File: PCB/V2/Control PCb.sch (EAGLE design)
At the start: 33 parts, among them Q1 DMP2305U-7, Q2 BSS123, Q3 BSS123, U1 V_REG_317DPACK, U2 5ACFEW

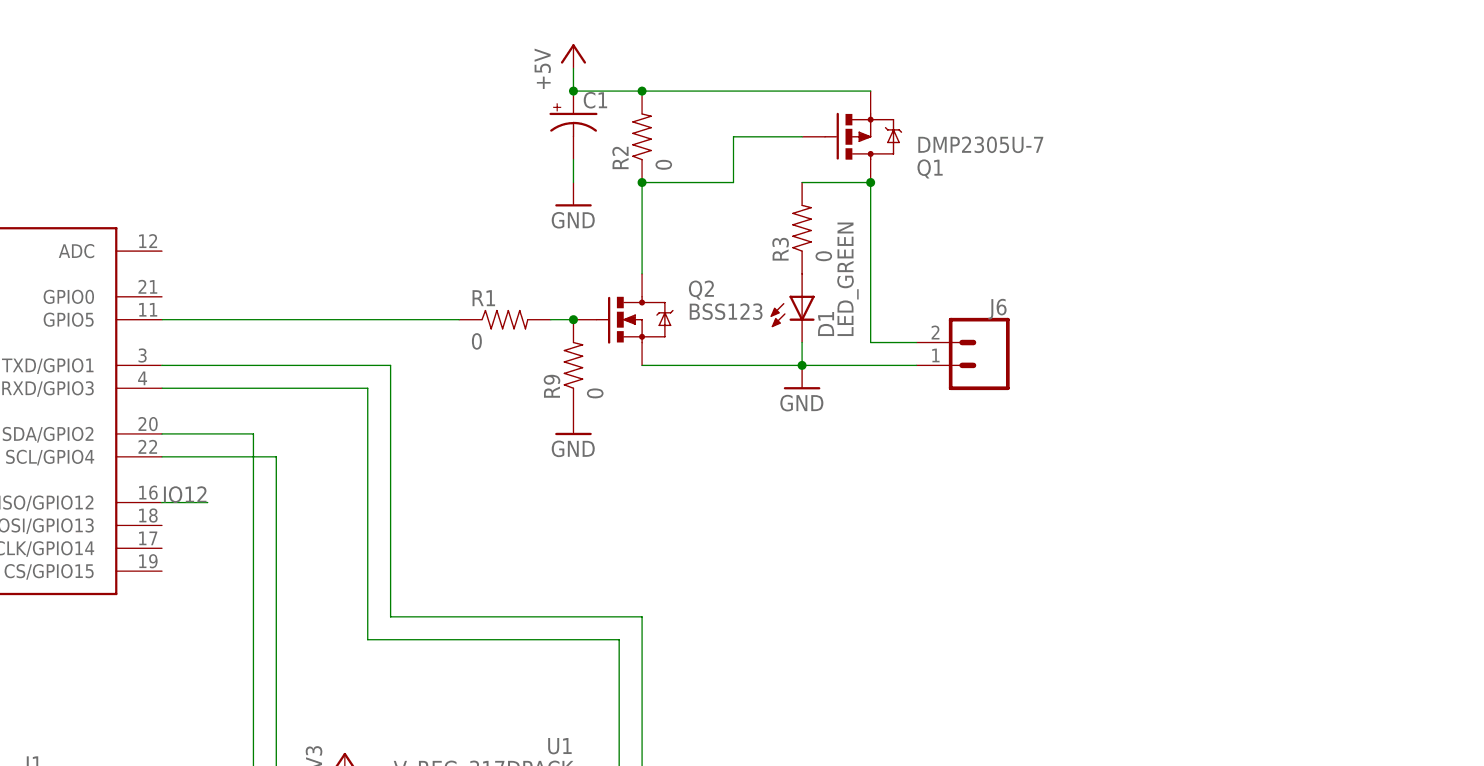
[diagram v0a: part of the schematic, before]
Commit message: Code + PCB stuff
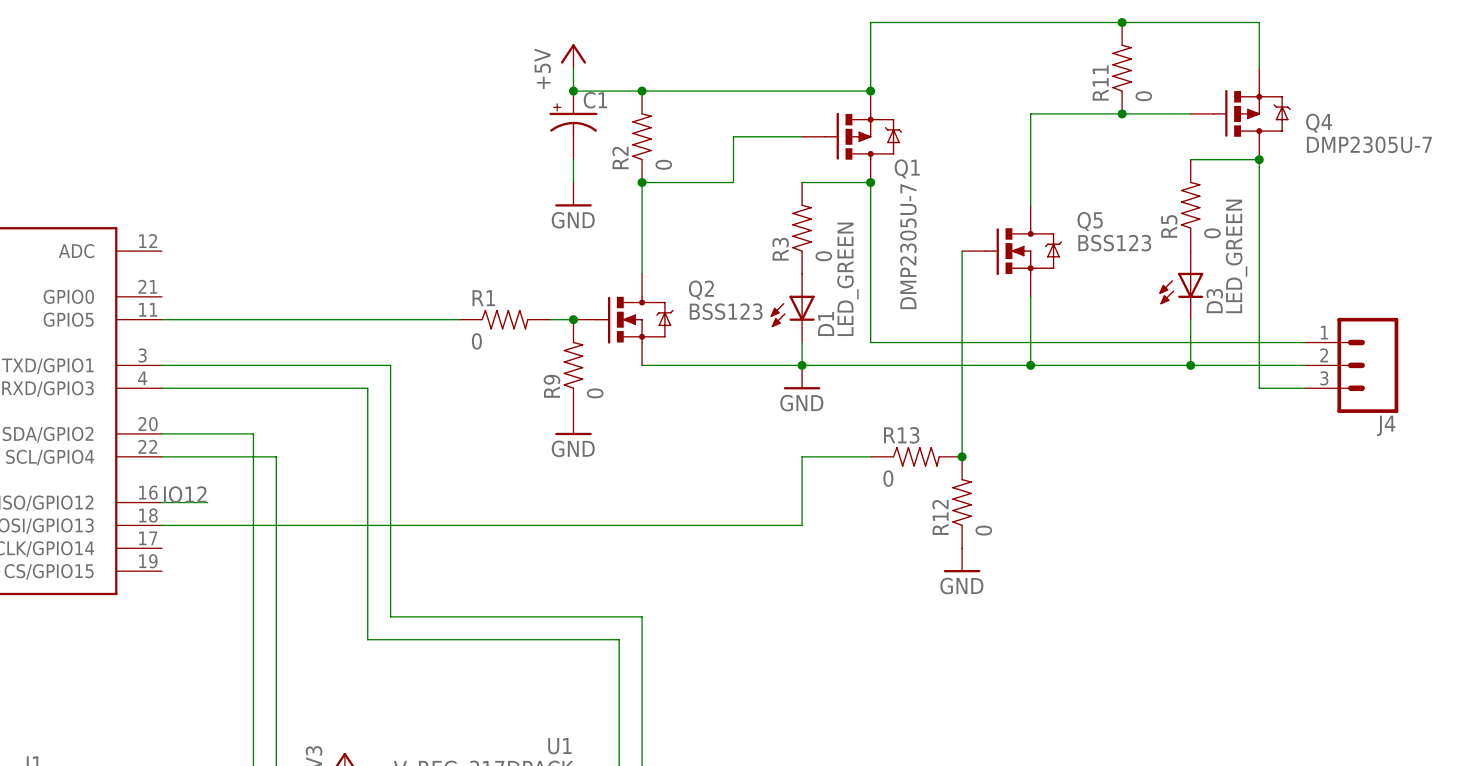
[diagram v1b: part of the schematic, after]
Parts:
- removed J6: (no value), SparkFun-Connectors:CONN_025MM
- added D3: LED_GREEN, RJC-2:LED_GREEN
- added J4: (no value), SparkFun-Connectors:CONN_03-SCREW-5MM
- added Q4: DMP2305U-7, RJC-2:MOS-P_DMP2305U-7
- added Q5: BSS123, RJC-2:MOS-N_BSS123
- added R11, R12, R13, R5: 0, RJC-2:RES_0_0805
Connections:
- new net N$16: J4.3, Q4.D, R5.2
- new net N$19: D3.A, R5.1
- new net N$20: Q4.G, Q5.D, R11.1
- new net N$21: R13.1, U$1.MOSI/GPIO13
- new net N$22: Q5.G, R12.2, R13.2
- net +5V: now also Q4.S, R11.2
- net GND: now also D3.C, J4.2, Q5.S, R12.1; no longer J6.1
- net N$6: now also J4.1; no longer J6.2
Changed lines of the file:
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@@
 <part name="GND6" library="supply1" library_urn="urn:adsk.eagle:library:371" deviceset="GND" device=""/>
 <part name="GND7" library="supply1" library_urn="urn:adsk.eagle:library:371" deviceset="GND" device=""/>
-<part name="J6" library="SparkFun-Connectors" library_urn="urn:adsk.eagle:library:513" deviceset="CONN_02" device="5MM" package3d_urn="urn:adsk.eagle:package:38044/1"/>
 <part name="R9" library="RJC-2" library_urn="urn:adsk.eagle:library:33162582" deviceset="RES" device="_0_0805" package3d_urn="urn:adsk.eagle:package:33163805/3" value="0"/>
 <part name="GND8" library="supply1" library_urn="urn:adsk.eagle:library:371" deviceset="GND" device=""/>
@@
 <part name="C2" library="SparkFun-Capacitors" library_urn="urn:adsk.eagle:library:510" deviceset="1000UF" device="-RADIAL-5MM-35V-20%-KIT" package3d_urn="urn:adsk.eagle:package:37421/1" value="470"/>
 <part name="C5" library="SparkFun-Capacitors" library_urn="urn:adsk.eagle:library:510" deviceset="1000UF" device="-RADIAL-5MM-35V-20%-KIT" package3d_urn="urn:adsk.eagle:package:37421/1" value="100"/>
+<part name="J4" library="SparkFun-Connectors" library_urn="urn:adsk.eagle:library:513" deviceset="CONN_03" device="-SCREW-5MM" package3d_urn="urn:adsk.eagle:package:38070/1"/>
+<part name="Q4" library="RJC-2" library_urn="urn:adsk.eagle:library:33162582" deviceset="MOS-P" device="_DMP2305U-7" package3d_urn="urn:adsk.eagle:package:33163661/2" value="DMP2305U-7"/>
+<part name="R5" library="RJC-2" library_urn="urn:adsk.eagle:library:33162582" deviceset="RES" device="_0_0805" package3d_urn="urn:adsk.eagle:package:33163805/3" value="0"/>
+<part name="D3" library="RJC-2" library_urn="urn:adsk.eagle:library:33162582" deviceset="LED" device="_GREEN" package3d_urn="urn:adsk.eagle:package:33163857/2"/>
+<part name="R11" library="RJC-2" library_urn="urn:adsk.eagle:library:33162582" deviceset="RES" device="_0_0805" package3d_urn="urn:adsk.eagle:package:33163805/3" value="0"/>
+<part name="Q5" library="RJC-2" library_urn="urn:adsk.eagle:library:33162582" deviceset="MOS-N" device="_BSS123" package3d_urn="urn:adsk.eagle:package:33163661/2" value="BSS123"/>
+<part name="R12" library="RJC-2" library_urn="urn:adsk.eagle:library:33162582" deviceset="RES" device="_0_0805" package3d_urn="urn:adsk.eagle:package:33163805/3" value="0"/>
+<part name="R13" library="RJC-2" library_urn="urn:adsk.eagle:library:33162582" deviceset="RES" device="_0_0805" package3d_urn="urn:adsk.eagle:package:33163805/3" value="0"/>
+<part name="GND10" library="supply1" library_urn="urn:adsk.eagle:library:371" deviceset="GND" device=""/>
 </parts>
 <sheets>
@@
 </instance>
 <instance part="Q1" gate="G$1" x="119.38" y="96.52" smashed="yes" rot="MR180">
-<attribute name="NAME" x="124.46" y="93.98" size="1.778" layer="95" rot="MR180"/>
-<attribute name="VALUE" x="124.46" y="96.52" size="1.778" layer="96" rot="MR180"/>
+<attribute name="NAME" x="121.92" y="93.98" size="1.778" layer="95" rot="MR180"/>
+<attribute name="VALUE" x="124.46" y="91.44" size="1.778" layer="96" rot="MR270"/>
 </instance>
 <instance part="Q2" gate="G$1" x="93.98" y="76.2" smashed="yes">
@@
 <attribute name="VALUE" x="109.22" y="66.04" size="1.778" layer="96"/>
 </instance>
-<instance part="J6" gate="G$1" x="132.08" y="71.12" smashed="yes" rot="MR0">
-<attribute name="VALUE" x="134.62" y="66.294" size="1.778" layer="96" font="vector" rot="MR0"/>
-<attribute name="NAME" x="134.62" y="76.708" size="1.778" layer="95" font="vector" rot="MR0"/>
-</instance>
 <instance part="R9" gate="G$1" x="86.36" y="71.12" smashed="yes" rot="R90">
 <attribute name="NAME" x="84.8614" y="67.31" size="1.778" layer="95" rot="R90"/>
@@
 <attribute name="NAME" x="89.916" y="-17.145" size="1.778" layer="95" font="vector"/>
 <attribute name="VALUE" x="89.916" y="-21.971" size="1.778" layer="96" font="vector"/>
+</instance>
+<instance part="J4" gate="J$1" x="175.26" y="71.12" smashed="yes" rot="R180">
+<attribute name="VALUE" x="177.8" y="78.486" size="1.778" layer="96" font="vector" rot="R180"/>
+<attribute name="NAME" x="177.8" y="65.532" size="1.778" layer="95" font="vector" rot="R180"/>
+</instance>
+<instance part="Q4" gate="G$1" x="162.56" y="99.06" smashed="yes" rot="MR180">
+<attribute name="NAME" x="167.64" y="99.06" size="1.778" layer="95" rot="MR180"/>
+<attribute name="VALUE" x="167.64" y="96.52" size="1.778" layer="96" rot="MR180"/>
+</instance>
+<instance part="R5" gate="G$1" x="154.94" y="88.9" smashed="yes" rot="R90">
+<attribute name="NAME" x="153.4414" y="85.09" size="1.778" layer="95" rot="R90"/>
+<attribute name="VALUE" x="158.242" y="85.09" size="1.778" layer="96" rot="R90"/>
+</instance>
+<instance part="D3" gate="G$1" x="154.94" y="78.74" smashed="yes">
+<attribute name="NAME" x="158.496" y="76.708" size="1.778" layer="95" rot="R90"/>
+<attribute name="VALUE" x="160.655" y="76.708" size="1.778" layer="96" rot="R90"/>
+</instance>
+<instance part="R11" gate="G$1" x="147.32" y="104.14" smashed="yes" rot="R90">
+<attribute name="NAME" x="145.8214" y="100.33" size="1.778" layer="95" rot="R90"/>
+<attribute name="VALUE" x="150.622" y="100.33" size="1.778" layer="96" rot="R90"/>
+</instance>
+<instance part="Q5" gate="G$1" x="137.16" y="83.82" smashed="yes">
+<attribute name="NAME" x="142.24" y="86.36" size="1.778" layer="95"/>
+<attribute name="VALUE" x="142.24" y="83.82" size="1.778" layer="96"/>
+</instance>
+<instance part="R12" gate="G$1" x="129.54" y="55.88" smashed="yes" rot="R90">
+<attribute name="NAME" x="128.0414" y="52.07" size="1.778" layer="95" rot="R90"/>
+<attribute name="VALUE" x="132.842" y="52.07" size="1.778" layer="96" rot="R90"/>
+</instance>
+<instance part="R13" gate="G$1" x="124.46" y="60.96" smashed="yes">
+<attribute name="NAME" x="120.65" y="62.4586" size="1.778" layer="95"/>
+<attribute name="VALUE" x="120.65" y="57.658" size="1.778" layer="96"/>
+</instance>
+<instance part="GND10" gate="1" x="129.54" y="48.26" smashed="yes">
+<attribute name="VALUE" x="127" y="45.72" size="1.778" layer="96"/>
 </instance>
 </instances>
@@
 <junction x="111.76" y="71.12"/>
 <pinref part="GND7" gate="1" pin="GND"/>
-<pinref part="J6" gate="G$1" pin="1"/>
-<wire x1="124.46" y1="71.12" x2="111.76" y2="71.12" width="0.1524" layer="91"/>
+<wire x1="167.64" y1="71.12" x2="154.94" y2="71.12" width="0.1524" layer="91"/>
+<pinref part="J4" gate="J$1" pin="2"/>
+<pinref part="D3" gate="G$1" pin="C"/>
+<wire x1="154.94" y1="71.12" x2="137.16" y2="71.12" width="0.1524" layer="91"/>
+<wire x1="137.16" y1="71.12" x2="111.76" y2="71.12" width="0.1524" layer="91"/>
+<wire x1="154.94" y1="76.2" x2="154.94" y2="71.12" width="0.1524" layer="91"/>
+<junction x="154.94" y="71.12"/>
+<pinref part="Q5" gate="G$1" pin="S"/>
+<wire x1="137.16" y1="78.74" x2="137.16" y2="71.12" width="0.1524" layer="91"/>
+<junction x="137.16" y="71.12"/>
 </segment>
 <segment>
@@
 <pinref part="GND9" gate="1" pin="GND"/>
 <wire x1="-7.62" y1="81.28" x2="-7.62" y2="78.74" width="0.1524" layer="91"/>
+</segment>
+<segment>
+<pinref part="R12" gate="G$1" pin="1"/>
+<pinref part="GND10" gate="1" pin="GND"/>
 </segment>
 </net>
@@
 <wire x1="93.98" y1="101.6" x2="119.38" y2="101.6" width="0.1524" layer="91"/>
 <junction x="93.98" y="101.6"/>
+<wire x1="119.38" y1="101.6" x2="119.38" y2="109.22" width="0.1524" layer="91"/>
+<wire x1="119.38" y1="109.22" x2="147.32" y2="109.22" width="0.1524" layer="91"/>
+<junction x="119.38" y="101.6"/>
+<pinref part="Q4" gate="G$1" pin="S"/>
+<wire x1="147.32" y1="109.22" x2="162.56" y2="109.22" width="0.1524" layer="91"/>
+<wire x1="162.56" y1="109.22" x2="162.56" y2="104.14" width="0.1524" layer="91"/>
+<pinref part="R11" gate="G$1" pin="2"/>
+<junction x="147.32" y="109.22"/>
 </segment>
 <segment>
@@
 <wire x1="119.38" y1="91.44" x2="119.38" y2="73.66" width="0.1524" layer="91"/>
 <junction x="119.38" y="91.44"/>
-<pinref part="J6" gate="G$1" pin="2"/>
-<wire x1="119.38" y1="73.66" x2="124.46" y2="73.66" width="0.1524" layer="91"/>
+<wire x1="119.38" y1="73.66" x2="167.64" y2="73.66" width="0.1524" layer="91"/>
+<pinref part="J4" gate="J$1" pin="1"/>
 </segment>
 </net>
@@
 </segment>
 </net>
+<net name="N$16" class="0">
+<segment>
+<pinref part="Q4" gate="G$1" pin="D"/>
+<wire x1="162.56" y1="93.98" x2="162.56" y2="68.58" width="0.1524" layer="91"/>
+<pinref part="J4" gate="J$1" pin="3"/>
+<wire x1="162.56" y1="68.58" x2="167.64" y2="68.58" width="0.1524" layer="91"/>
+<pinref part="R5" gate="G$1" pin="2"/>
+<wire x1="154.94" y1="93.98" x2="162.56" y2="93.98" width="0.1524" layer="91"/>
+<junction x="162.56" y="93.98"/>
+</segment>
+</net>
+<net name="N$19" class="0">
+<segment>
+<pinref part="R5" gate="G$1" pin="1"/>
+<pinref part="D3" gate="G$1" pin="A"/>
+</segment>
+</net>
+<net name="N$20" class="0">
+<segment>
+<pinref part="R11" gate="G$1" pin="1"/>
+<pinref part="Q4" gate="G$1" pin="G"/>
+<wire x1="147.32" y1="99.06" x2="154.94" y2="99.06" width="0.1524" layer="91"/>
+<pinref part="Q5" gate="G$1" pin="D"/>
+<wire x1="137.16" y1="88.9" x2="137.16" y2="99.06" width="0.1524" layer="91"/>
+<wire x1="137.16" y1="99.06" x2="147.32" y2="99.06" width="0.1524" layer="91"/>
+<junction x="147.32" y="99.06"/>
+</segment>
+</net>
+<net name="N$22" class="0">
+<segment>
+<pinref part="R12" gate="G$1" pin="2"/>
+<pinref part="R13" gate="G$1" pin="2"/>
+<pinref part="Q5" gate="G$1" pin="G"/>
+<wire x1="129.54" y1="83.82" x2="129.54" y2="60.96" width="0.1524" layer="91"/>
+<junction x="129.54" y="60.96"/>
+</segment>
+</net>
+<net name="N$21" class="0">
+<segment>
+<pinref part="U$1" gate="G$1" pin="MOSI/GPIO13"/>
+<wire x1="40.64" y1="53.34" x2="111.76" y2="53.34" width="0.1524" layer="91"/>
+<wire x1="111.76" y1="53.34" x2="111.76" y2="60.96" width="0.1524" layer="91"/>
+<pinref part="R13" gate="G$1" pin="1"/>
+<wire x1="111.76" y1="60.96" x2="119.38" y2="60.96" width="0.1524" layer="91"/>
+</segment>
+</net>
